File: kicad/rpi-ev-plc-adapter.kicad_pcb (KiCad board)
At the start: 4 copper layers, 65.1 x 56.6 mm, 91 parts, among them J1 Raspberry_RPI, J10 socket, J2 Conn_01x06, J3 header, J5 header, J6 Screw_Terminal_01x03, J7 Conn_01x03, J8 Conn_01x03, J9 socket, M1 I2PLCAMN-ISE-002-T, M2 supply-5Vto3V3_ebay-303262143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, M3 supply-5VtoPM12V_ebay-2530527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, Q1 AO3400, Q2 AO3401, Q3 AO3400, Q4 AO3401, SW1 push-button_ebay-183284526496, SW2 push-button_ebay-183284526496, SW3 SS-12D00G3, SW4 SS-12D00G3, SW5 dip-switch-6x2pos-smd-1.27mm, U1 LM224

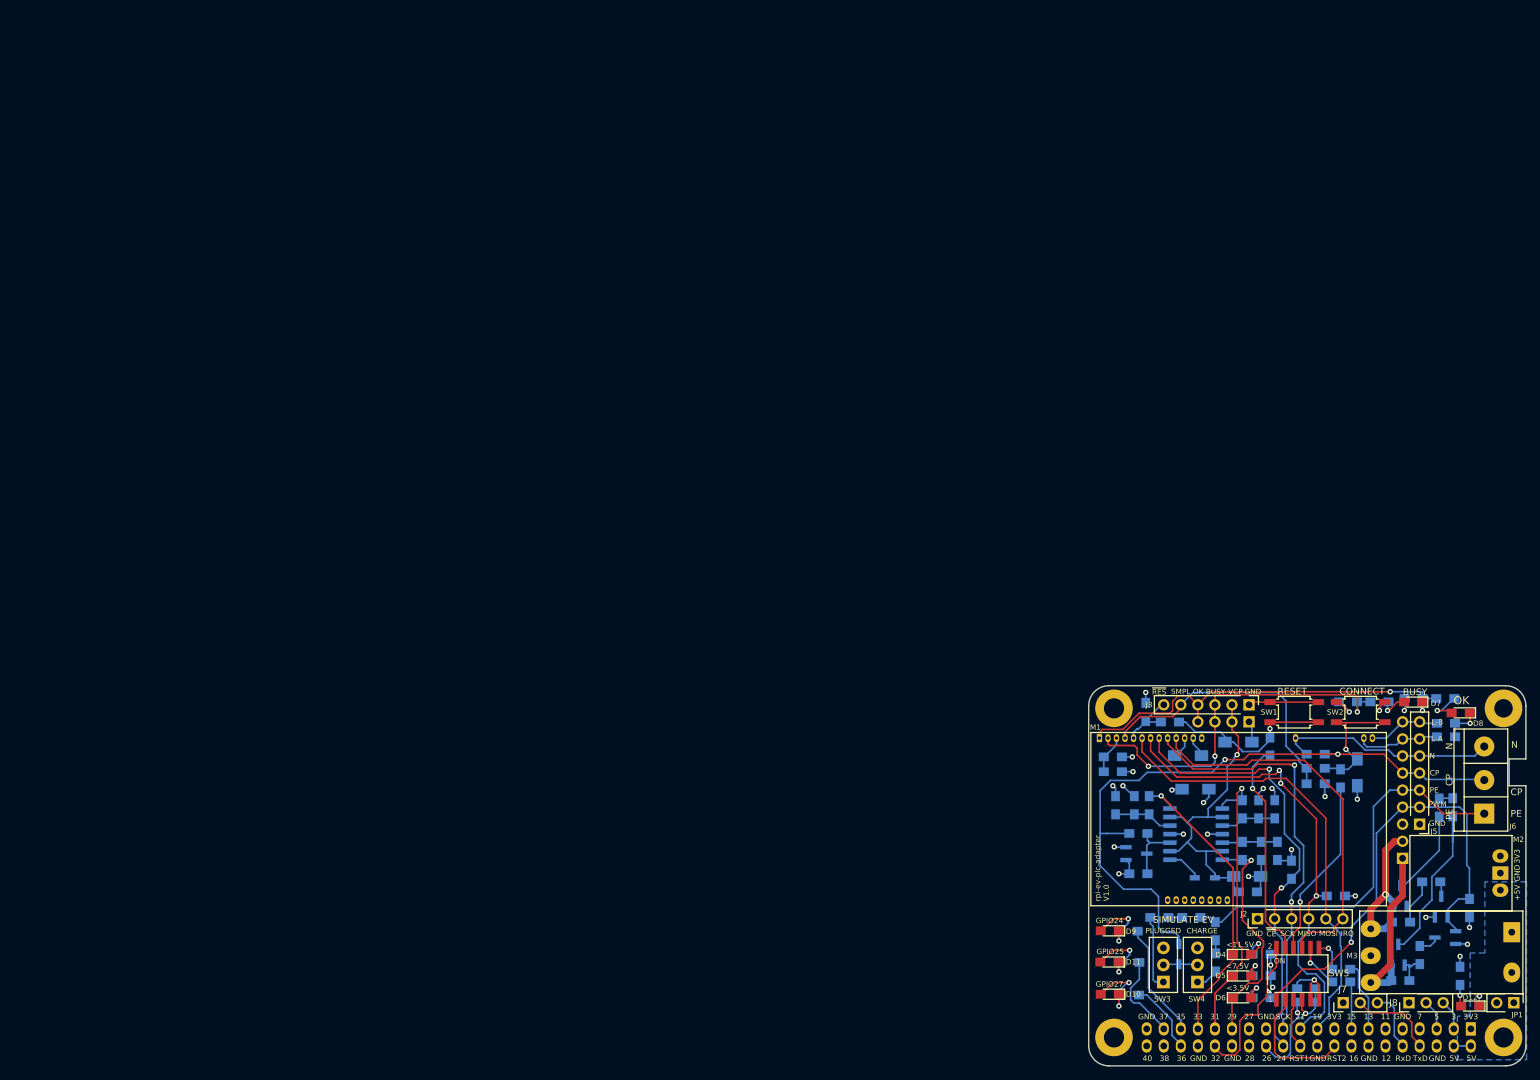
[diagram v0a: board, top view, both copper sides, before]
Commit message: ...
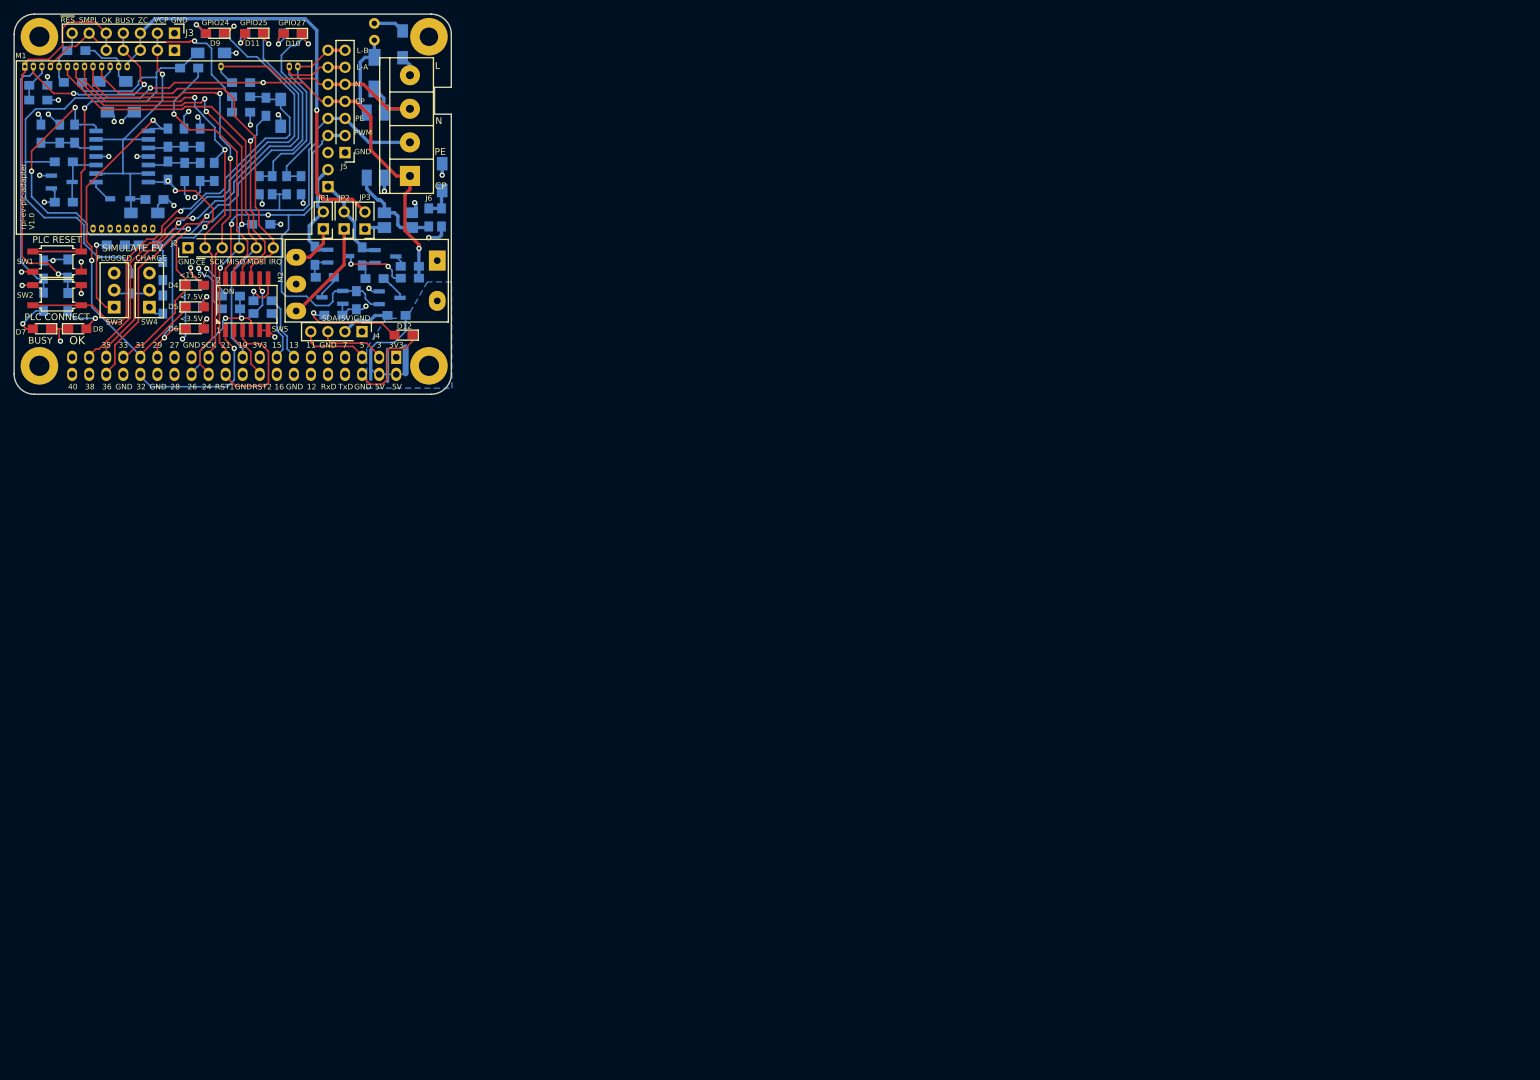
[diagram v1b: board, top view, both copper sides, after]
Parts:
- removed J7, J8: Conn_01x03, Project:idc-header-1x03-p2.54mm-vertical
- removed M3: supply-5VtoPM12V_ebay-253052736386, Project:5V-to-PM12V_ebay-253052736386
- added C6: 2.2n, Capacitors_THT:C_Disc_D3.8mm_W2.6mm_P2.50mm, B.Cu at (-3.26, -49.7)
- added C7: 220n, Project:c-1206-hand-soldering, B.Cu at (0.24, -21.5)
- added C8: 1u, Project:c-1206-hand-soldering, B.Cu at (6.84, -26.8)
- added C9: 1n, Project:c-1206-hand-soldering, B.Cu at (0.24, -19.3)
- added D13: 1N4007, Project:sma_hand-soldering, B.Cu at (-3.24, -42.3)
- added J4: header, Project:idc-header-1x04-p2.54mm-vertical, F.Cu at (-5.10, -3.82)
- added JP2: Jumper_NO_Small, Project:idc-header-1x02-p2.54mm-vertical, F.Cu at (-7.76, -19.1)
- added JP3: Jumper_NO_Small, Project:idc-header-1x02-p2.54mm-vertical, F.Cu at (-4.66, -19.1)
- added R52: 0R, Project:r-0805-hand-soldering, B.Cu at (0.05, -6.24)
- added R53: 0R, Project:r-0805-hand-soldering, B.Cu at (-18.5, -25.6)
- added R54: 0R, Project:r-0805-hand-soldering, B.Cu at (-16.3, -25.6)
- added R55: 820K, Project:r-1206-hand-soldering, B.Cu at (0.94, -46.6)
- added R56: 100R, Project:r-0805-hand-soldering, B.Cu at (6.74, -20.8)
- added R57: 39K, Project:r-0805-hand-soldering, B.Cu at (4.84, -20.8)
- added U2: PC817C, Project:sop-4-pc817, B.Cu at (-3.12, -31.6)
- J3: footprint Project:idc-header-1x06-p2.54mm-vertical -> Project:idc-header-1x07-p2.54mm-vertical
- J6: value Screw_Terminal_01x03 -> Screw_Terminal_01x04; footprint Project:screw-terminal-230v-16a-5mm-3pin -> Project:screw-terminal-230v-16a-5mm-4pin
- J9: footprint Project:idc-socket-1x04-p2.54mm-vertical -> Project:idc-socket-vertical-2.54mm_1x05
- M2: value supply-5Vto3V3_ebay-303262143289 -> supply-5VtoPM12V_ebay-253052736386; footprint Project:dc-dc-buck-converter-5v-to-3.3v-2a -> Project:5V-to-PM12V_ebay-253052736386
- R40, R41: value 0R -> 1G
- moved D8 213.8 mm to (-47.5, -4.25), turned to 0 degrees
- moved R45 213.4 mm to (-48.9, -8.22), turned to 270 degrees
- moved D7 211.6 mm to (-52.8, -4.25)
- moved JP1 211.4 mm to (-10.9, -19.1), turned to 180 degrees
- moved R44 210.4 mm to (-48.9, -13.2), turned to 270 degrees
- moved R43 207.6 mm to (-52.5, -8.27), turned to 270 degrees
- moved R42 204.6 mm to (-52.5, -13.1), turned to 270 degrees
- moved SW2 203.8 mm to (-50.5, -9.25)
- moved SW1 196.0 mm to (-50.5, -14.2), turned to 180 degrees
- moved R40 194.8 mm to (-20.4, -25.6), turned to 270 degrees
- moved R51 194.5 mm to (-9.36, -6.27), turned to 0 degrees
- moved R19 192.7 mm to (-36.0, -23.5)
- moved C5 191.6 mm to (-37.5, -21.5)
- moved R36 191.5 mm to (-24.6, -9.12)
- moved R1 191.1 mm to (-27.1, -27.6), turned to 90 degrees
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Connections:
- net Net-(J1-Pad35) renamed /GPIO24
- net Net-(J1-Pad36) renamed /GPIO27
- net Net-(J1-Pad37) renamed /GPIO25
- J1 pad 1: /3V3PI -> +3V3
- J1 pad 10: Net-(J1-Pad10) -> (no net)
- J1 pad 17: /3V3PI -> +3V3
- J1 pad 3: Net-(J1-Pad3) -> /SDA1
- J1 pad 5: Net-(J1-Pad5) -> /SCL1
- J1 pad 8: Net-(J1-Pad8) -> (no net)
- J3 pad 3: /CONNECTING -> /ZERODET
- J3 pad 4: /CONNECTED -> /CONNECTING
- J3 pad 5: /SMPLCONN -> /CONNECTED
- J3 pad 6: /~RESET -> /SMPLCONN
- J6 pad 1: /PE -> /CP
- J6 pad 2: /CP -> /PE
- J9 pad 3: /CONNECTING -> /ZERODET
- J9 pad 4: /CONNECTED -> /CONNECTING
- JP1 pad 1: +3V3 -> /M-12V
- JP1 pad 2: /3V3PI -> -12V
- M1 pad 13: (no net) -> /ZERODET
- M2 pad 1: +5V -> GND
- M2 pad 2: GND -> +5V
- M2 pad 3: +3V3 -> /M+12V
- SW5 pad 1: /PWM -> Net-(J1-Pad32)
- SW5 pad 2: Net-(J1-Pad32) -> /PWM
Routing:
- net /ZERODET: track 0.00 -> 66.2 mm, vias 0 -> 1
- net /GPIO27: track 10.8 -> 70.0 mm, vias 0 -> 1
- net /GPIO25: track 13.0 -> 68.7 mm, vias 0 -> 1
- net /GPIO24: track 17.2 -> 68.7 mm, vias 0 -> 1
- net Net-(C3-Pad1): track 19.2 -> 67.6 mm
- net Net-(C2-Pad1): track 27.8 -> 64.6 mm
- net /Control-Pilot/VCPLT11V5: track 45.5 -> 74.1 mm, vias 1 -> 3
- net +5V: track 3.04 -> 29.0 mm
- net Net-(Q2-Pad3): track 26.7 -> 1.76 mm
- net /CP: track 103.3 -> 125.2 mm, vias 2 -> 3
- net /L-A: track 12.5 -> 32.4 mm
- net /L-B: track 10.7 -> 29.1 mm
- net /M+12V: track 0.00 -> 15.3 mm
- net /Control-Pilot/VCPLT7V5: track 43.8 -> 58.8 mm, vias 1 -> 2
- net Net-(C7-Pad1): track 0.00 -> 14.9 mm
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- removed copper zone on In1.Cu, net /3V3PI
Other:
- board text added: "(5V)"
- board text added: "L"
- board text added: "PLC CONNECT"
- board text added: "PLC RESET"
- board text added: "SDA"
- board text added: "ZC"
- board text removed: "CONNECT"
- board text removed: "RESET"
